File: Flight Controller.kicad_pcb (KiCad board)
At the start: 4 copper layers, 39.5 x 39.5 mm, 151 parts, among them IC2 AT7456E, J1 Conn_01x08_MountingPin, J2 USB_C_Receptacle_USB2.0_14P, Q2 BC817W, SW1 SW_SPST, U1 AT32F435RGT7, U2 LMR51430, U3 BMP280, U4 SPX3819M5-L-3-3, U5 LMR51430, U6 W25Q128JVSIQ TR, U7 ICM-42688-P, U8 SPX3819M5-L-3-3, Y1 8M, Y2 27M

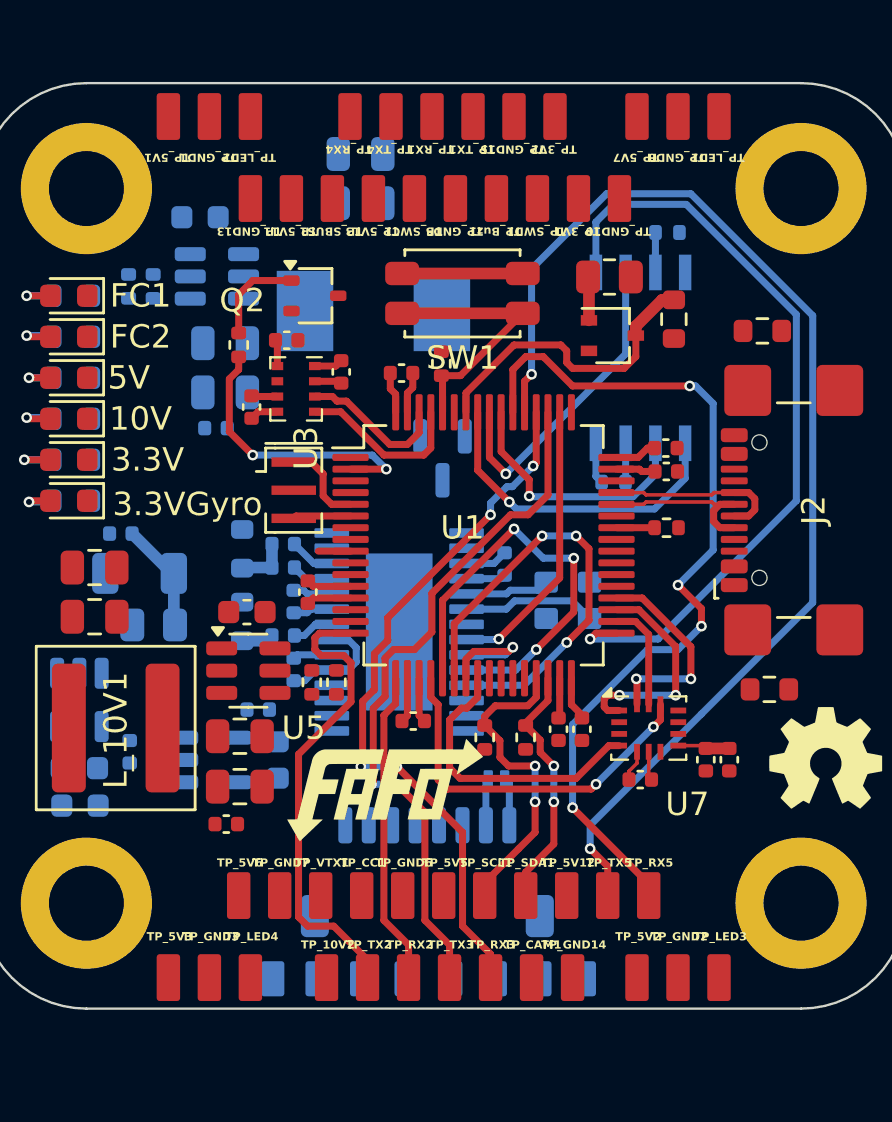
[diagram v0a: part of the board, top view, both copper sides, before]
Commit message: Layout Updates
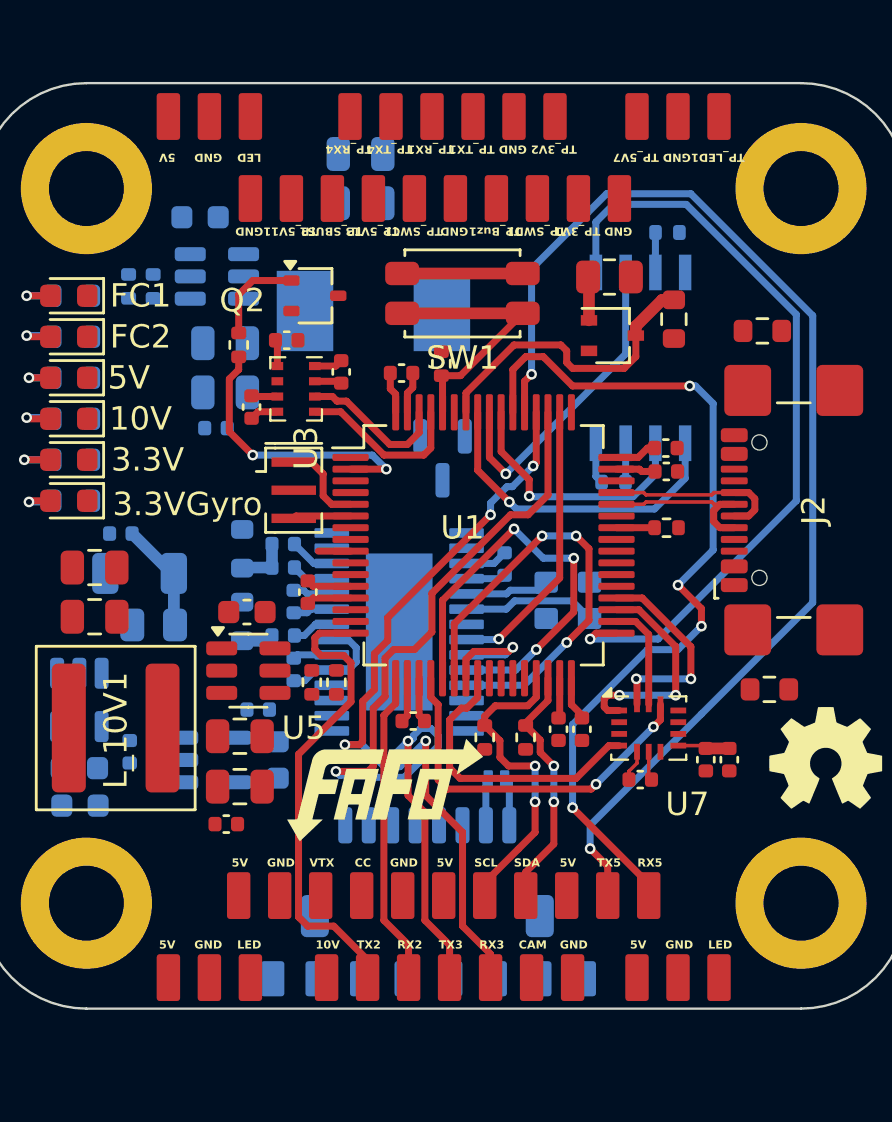
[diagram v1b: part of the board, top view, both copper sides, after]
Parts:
- renumbered TP_10V2 to 10V, TP_5V12 to 5V, TP_5V6 to 5V, TP_5V3 to 5V, TP_5V2 to 5V, TP_5V1 to 5V, TP_5V5 to 5V, TP_CAM1 to CAM, TP_CC1 to CC, TP_GND14 to GND, TP_GND10 to GND, TP_GND15 to GND, TP_GND1 to GND, TP_GND3 to GND, TP_GND5 to GND, TP_GND6 to GND, TP_GND2 to GND, TP_GND8 to GND, TP_GND13 to GND, TP_GND7 to GND, TP_LED4 to LED, TP_LED3 to LED, TP_LED2 to LED, TP_RX2 to RX2, TP_RX3 to RX3, TP_RX5 to RX5, TP_SCL1 to SCL, TP_SDA1 to SDA, TP_TX2 to TX2, TP_TX3 to TX3, TP_TX5 to TX5, TP_VTX1 to VTX
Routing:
- net /UART3_TX: track 30.2 -> 40.7 mm
- net /UART3_RX: track 30.6 -> 33.6 mm
